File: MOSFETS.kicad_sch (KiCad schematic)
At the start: 18 parts, among them Q1 Q_NMOS_GDS, Q10 Q_NMOS_GDS, Q11 Q_NMOS_GDS, Q12 Q_NMOS_GDS, Q2 Q_NMOS_GDS, Q3 Q_NMOS_GDS, Q4 Q_NMOS_GDS, Q5 Q_NMOS_GDS, Q6 Q_NMOS_GDS, Q7 Q_NMOS_GDS, Q8 Q_NMOS_GDS, Q9 Q_NMOS_GDS

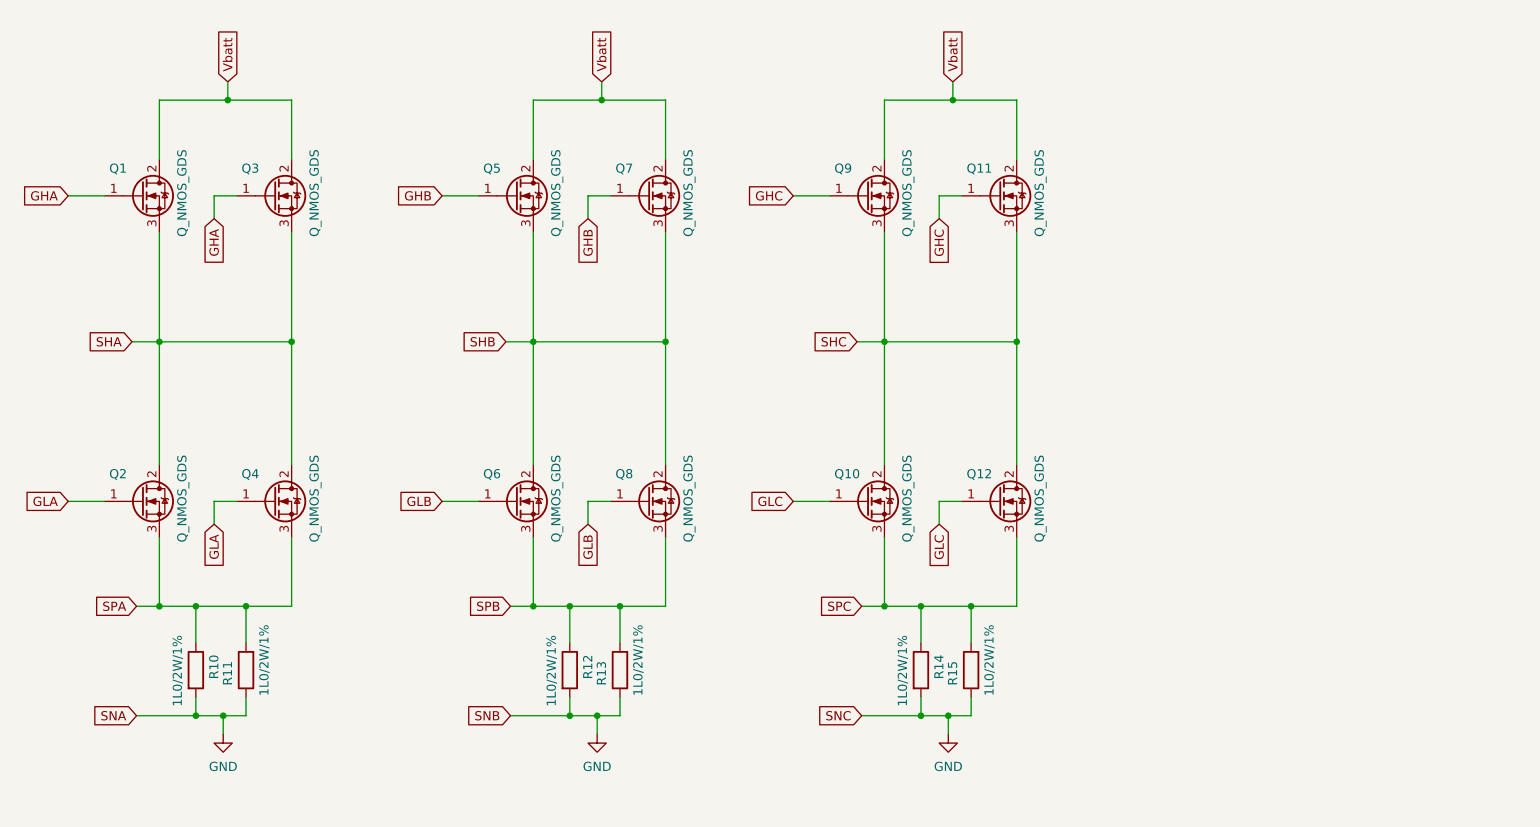
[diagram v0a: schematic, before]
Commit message: Updated Schematics and worked on board layout
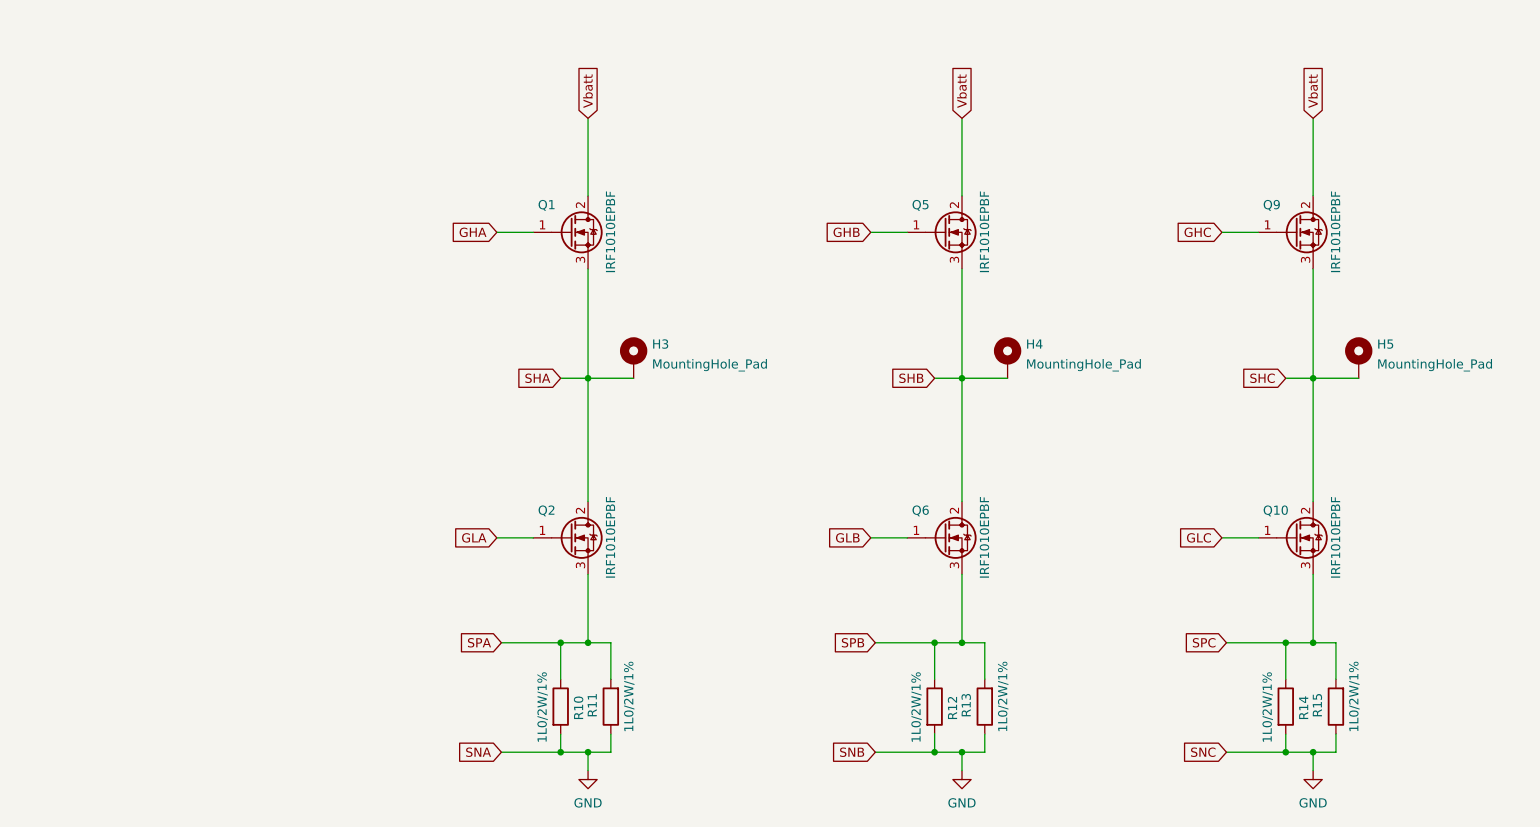
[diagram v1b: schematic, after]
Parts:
- removed Q11, Q12, Q3, Q4, Q7, Q8: Q_NMOS_GDS, symbol Device:Q_NMOS_GDS
- added H3, H4, H5: MountingHole_Pad, MountingHole:MountingHole_2.7mm, symbol Mechanical:MountingHole_Pad
- Q1, Q10, Q2, Q5, Q6, Q9: value Q_NMOS_GDS -> IRF1010EPBF; footprint (none) -> Package_TO_SOT_THT:TO-220-3_Horizontal_TabUp; MPN IRF60R217 -> IRF1010EPBF; Supplier_PN IRF60R217CT-ND -> IRF1010EPBF-ND
- R10, R11, R12, R13, R14, R15: footprint (none) -> Resistor_SMD:R_2512_6332Metric
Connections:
- net SHA: now also H3.1
- net SHB: now also H4.1
- net SHC: now also H5.1
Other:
- moved on the sheet: Q1, Q10, Q2, Q5, Q6, Q9, R10, R11, R12, R13, R14, R15
